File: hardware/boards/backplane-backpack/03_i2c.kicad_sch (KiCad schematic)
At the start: 33 parts, among them J3 I2C CH0 (TBD), J4 I2C CH1 (TBD), J5 I2C CH2 (TBD), J6 I2C CH3 (TBD), J7 I2C CH4 (TBD), J8 I2C CH5 (TBD), U2 TCA9548APWR

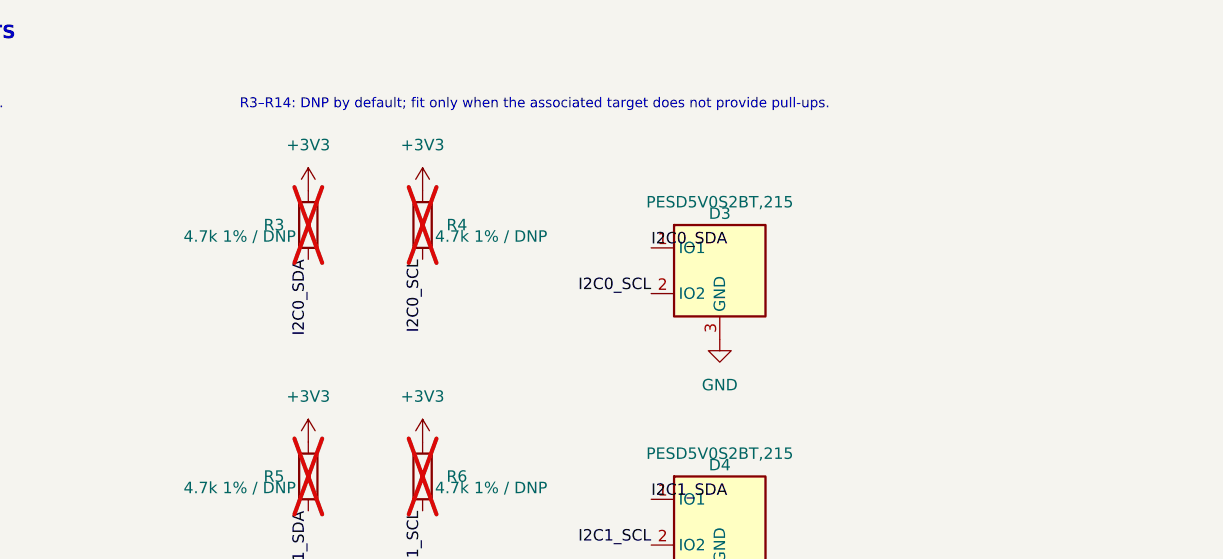
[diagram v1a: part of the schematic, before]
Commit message: chore: checkpoint workspace changes
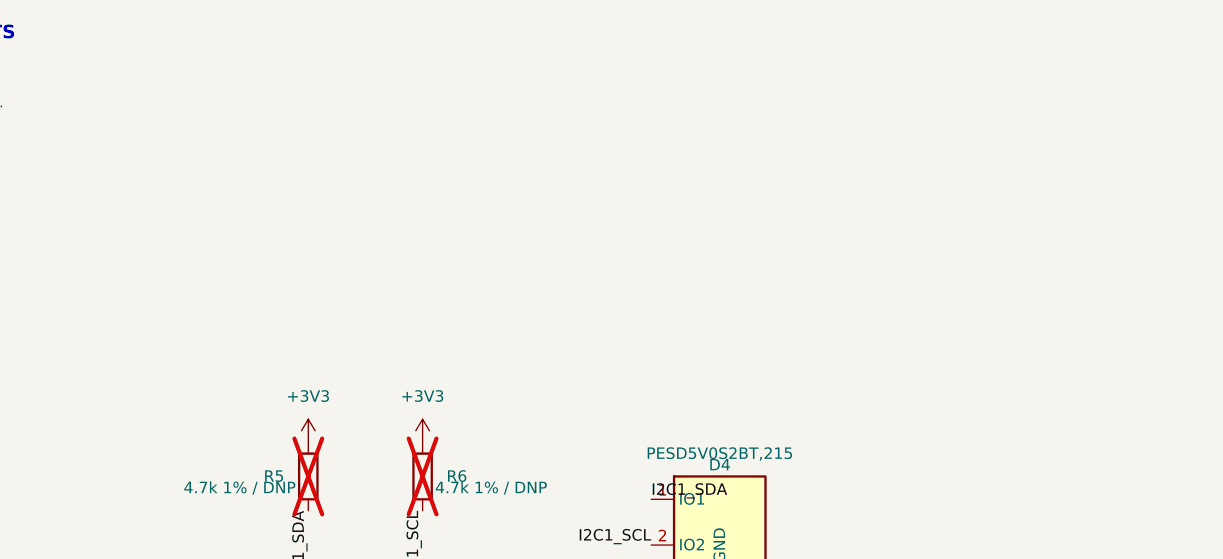
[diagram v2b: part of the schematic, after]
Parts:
- removed D3: PESD5V0S2BT,215, Package_TO_SOT_SMD:SOT-23, symbol backplane-backpack:PESD_Dual_SOT23
- removed R3, R4: 4.7k 1% / DNP, Resistor_SMD:R_0603_1608Metric, symbol Device:R
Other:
- note removed: "R3–R14: DNP by default; fit only when the associated target does not provide pull-ups."
